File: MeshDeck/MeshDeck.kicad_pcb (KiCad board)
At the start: 4 copper layers, 88.9 x 121.6 mm, 234 parts, among them CN1 ATGM336H-6N-74, J1 Conn_01x03_MountingPin, SW1 4*4*1.7, SW10 4*4*1.7, SW11 4*4*1.7, SW12 4*4*1.7, SW13 4*4*1.7, SW14 4*4*1.7, SW15 4*4*1.7, SW16 4*4*1.7, SW17 4*4*1.7, SW18 4*4*1.7, SW19 4*4*1.7, SW2 4*4*1.7, SW20 4*4*1.7, SW21 4*4*1.7, SW22 4*4*1.7, SW23 4*4*1.7, SW24 4*4*1.7, SW25 4*4*1.7, SW26 4*4*1.7, SW27 4*4*1.7, SW28 4*4*1.7, SW29 4*4*1.7, SW3 SKHHLVA010, SW30 4*4*1.7, SW31 4*4*1.7, SW32 4*4*1.7, SW33 4*4*1.7, SW34 4*4*1.7, SW35 4*4*1.7, SW36 4*4*1.7, SW37 4*4*1.7, SW38 4*4*1.7, SW39 4*4*1.7, SW4 4*4*1.7, SW5 4*4*1.7, SW6 4*4*1.7, SW7 4*4*1.7, SW8 4*4*1.7, SW9 4*4*1.7, U1 ESP32-S3-WROOM-1U-N16R8, U10 ABM8-272-T3_C20625731, U2 SX1262S8S+T-X1, U3 TPS6282533DMQR, U4 BQ24074RGTR, U5 RN32768114, U7 CD4013BM, U8 RP2040, U9 W25Q128JVSIQTR

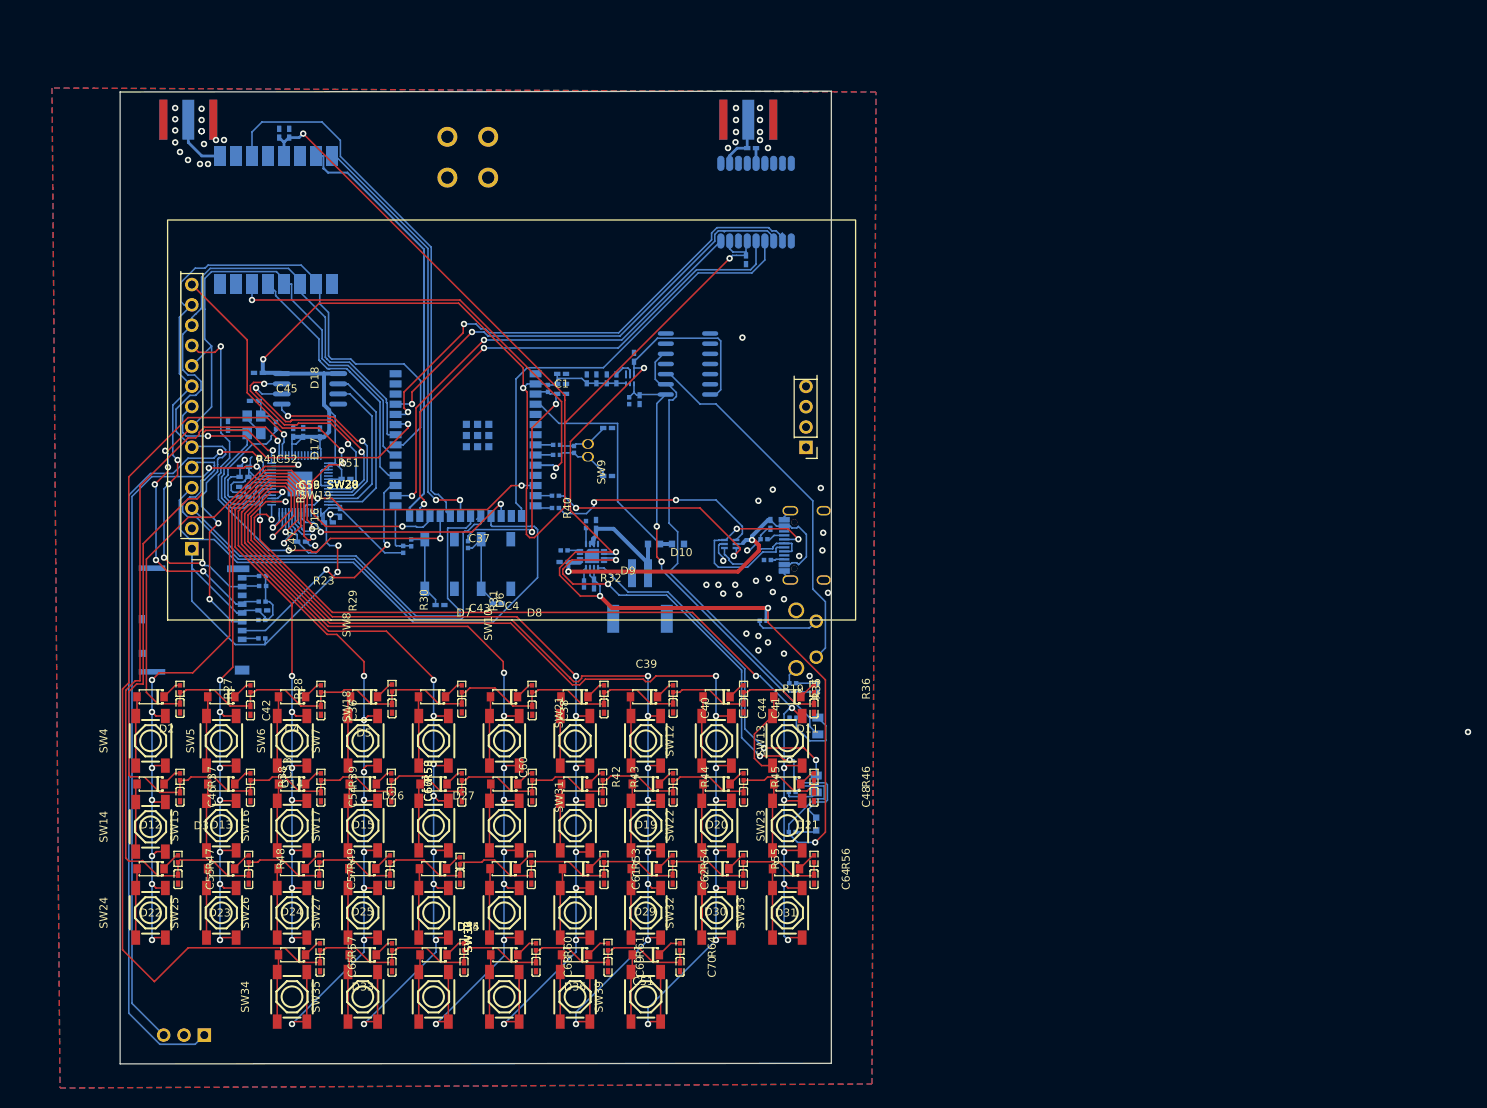
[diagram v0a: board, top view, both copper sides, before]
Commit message: Finished PCB
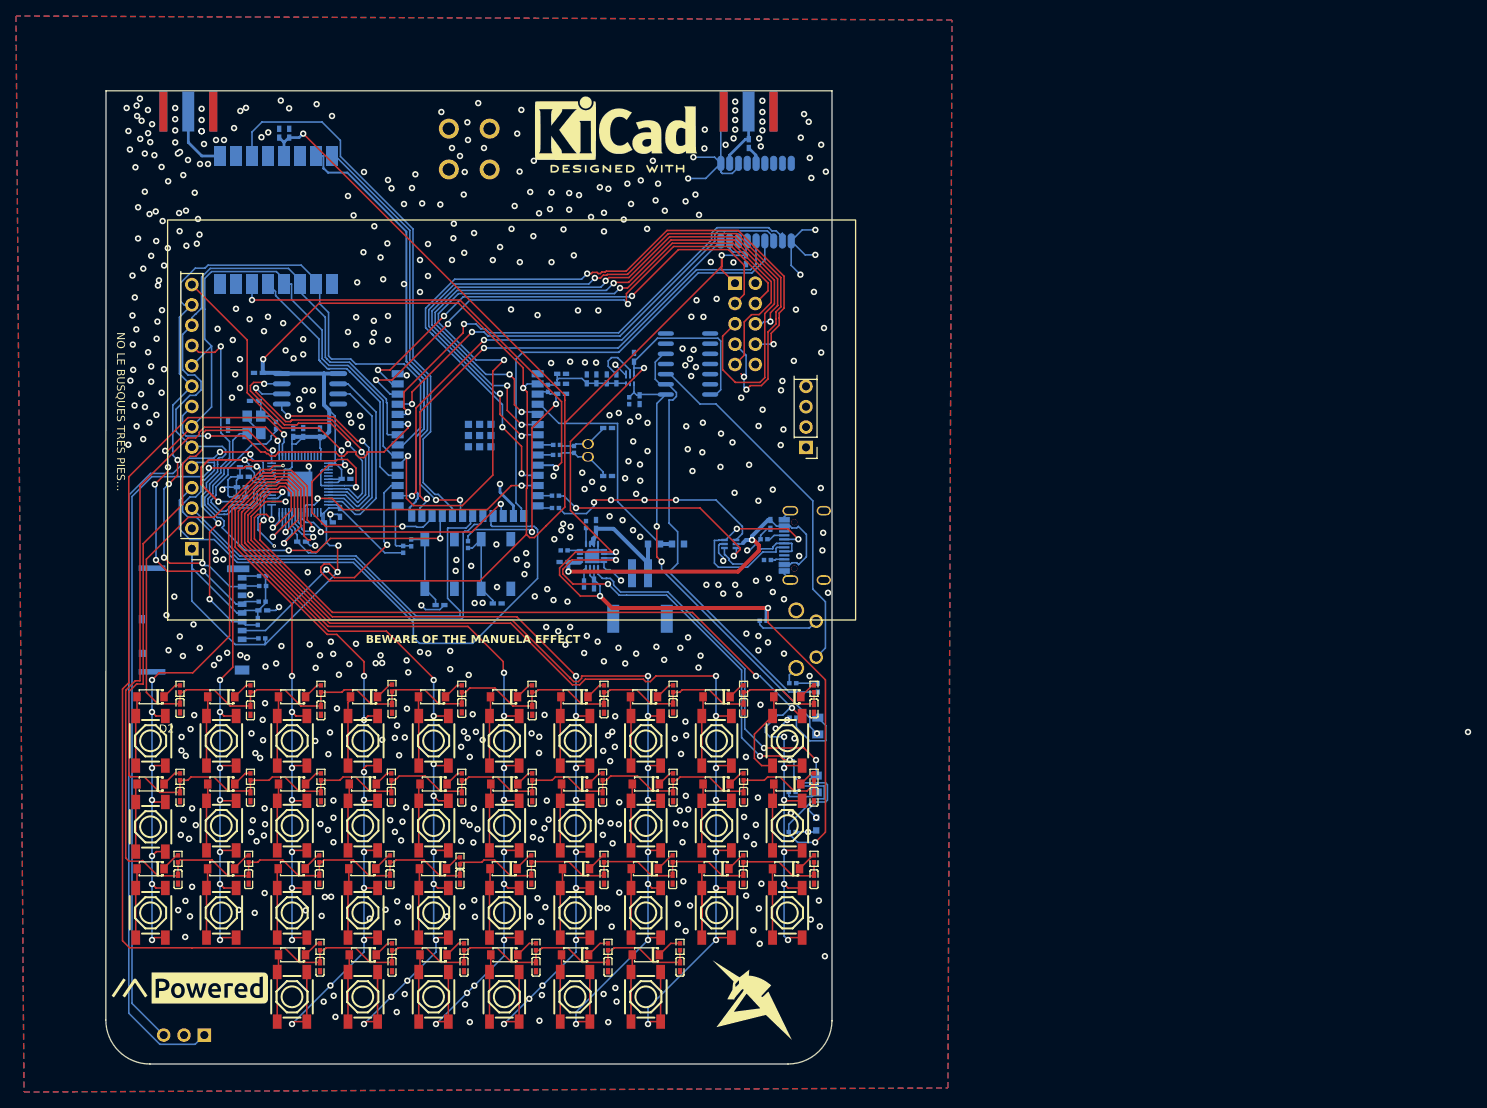
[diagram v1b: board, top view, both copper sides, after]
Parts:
- added G***: LOGO, LOGO, F.Cu at (105.0, 143.0)
- added G***: LOGO, LOGO, F.Cu at (175.5, 144.5)
- added G***: LOGO, LOGO, B.Cu at (129.8, 35.2)
- added G***: LOGO, LOGO, B.Cu at (153.4, 35.2)
- added G***: LOGO, LOGO, B.Cu at (140.1, 114.0)
- added J2: Conn_02x05_Odd_Even, Connector_PinSocket_2.54mm:PinSocket_2x05_P2.54mm_Horizontal, B.Cu at (173.4, 54.9)
- added REF**: KiCad-Logo2_8mm_SilkScreen, Symbol:KiCad-Logo2_8mm_SilkScreen, F.Cu at (158.5, 35.5)
- added REF**: OSHW-Logo2_36.5x30mm_SilkScreen, Symbol:OSHW-Logo2_36.5x30mm_SilkScreen, B.Cu at (140.1, 144.0)
- moved C29 1.34 mm to (111.7, 80.4)
- moved C22 1.26 mm to (112.0, 79.1)
- moved REF** 1.04 mm to (140.2, 38.1)
- moved RF2 1.02 mm to (175.1, 33.4)
- moved RF1 1.02 mm to (105.0, 33.4)
- moved L2 0.67 mm to (175.1, 37.5), turned to 90 degrees
- moved R23 0.54 mm to (113.7, 97.2), turned to -90 degrees
- moved C31 0.39 mm to (111.6, 81.6)
- moved U1 0.26 mm to (140.0, 75.1)
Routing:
- net /IO38: track 0.00 -> 106.4 mm, vias 0 -> 3
- net /IO7: track 0.00 -> 97.3 mm, vias 0 -> 5
- net /IO5: track 0.00 -> 94.2 mm, vias 0 -> 3
- net /IO18: track 0.00 -> 90.8 mm, vias 0 -> 4
- net /IO6: track 0.00 -> 78.8 mm, vias 0 -> 4
- net GND: track 30.0 -> 100.5 mm, vias 54 -> 544
- net /IO2: track 0.00 -> 65.8 mm, vias 0 -> 3
- net /IO1: track 0.00 -> 61.0 mm, vias 0 -> 3
- net /3V3: track 316.7 -> 356.2 mm
- net +1V1: track 16.9 -> 45.5 mm, vias 0 -> 3
- net /Keyboard/XIN: track 20.3 -> 24.7 mm
- net /Keyboard/ROW4: track 172.9 -> 168.8 mm
- net /Keyboard/ROW1: track 151.6 -> 147.7 mm
- net /TCH_CS: track 59.1 -> 62.8 mm
- net /Keyboard/XOUT: track 20.2 -> 23.8 mm
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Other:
- board size 88.9 x 121.6 mm -> 90.8 x 121.7 mm
- board text added: "+ -"
- board text added: "3V3"
- board text added: "BEWARE OF THE MANUELA EFFECT"
- board text added: "BOOT"
- board text added: "CHARGING LEDS"
- board text added: "DESIGNED IN SPAIN"
- board text added: "EA9353URE"
- board text added: "GND"
- board text added: "IO1"
- board text added: "IO18"
- board text added: "IO2"
- board text added: "IO38"
- board text added: "IO5"
- board text added: "IO6"
- board text added: "IO7"
- board text added: "NO LE BUSQUES TRES PIES..."
- board text added: "POWER LEDS"
- board text added: "RESET"
- board text added: "SWCLK"
- board text added: "SWD"
- board text added: "by ThePangel"
- board text removed: "${REFERENCE}"
